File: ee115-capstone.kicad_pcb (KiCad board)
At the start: 4 copper layers, 191 parts, among them J1 2171790001, J2 9V_BATTERY, J3 Conn_01x04_Pin, J5 Conn_01x03_Pin, J6 Conn_02x02_Odd_Even, Q1 PMOS, Q2 NMOS, Q3 NPN, Q4 AO3400A, Q5 AO3400A, Q6 NMOS, Q7 PNP, Q8 NPN, SW1 SW_Push, SW2 SW_Push, SW3 SW_Push, U1 OPA2140AIDR, U10 SN74LVC1G02DCKR (NOR), U11 SN74LVC1G02DCKR (NOR), U12 ALD1107PBL, U13 LD39150DT33-R, U14 SL78L05, U15 300P14-U, U16 OPA705PA, U17 MIC4605-2YM-TR, U18 OPA705PA, U19 OPA705PA, U2 CD4052BPWR, U20 AD8038, U21 MCP6571T-E/OT, U3 LM393DR, U4 ADG601BRMZ-REEL7, U5 ESP32-C3-WROOM-02-N4, U6 AP2112K-3.3, U7 MCP601T-E_OT, U8 MCP6571T-E/OT, U9 MCP6571T-E/OT

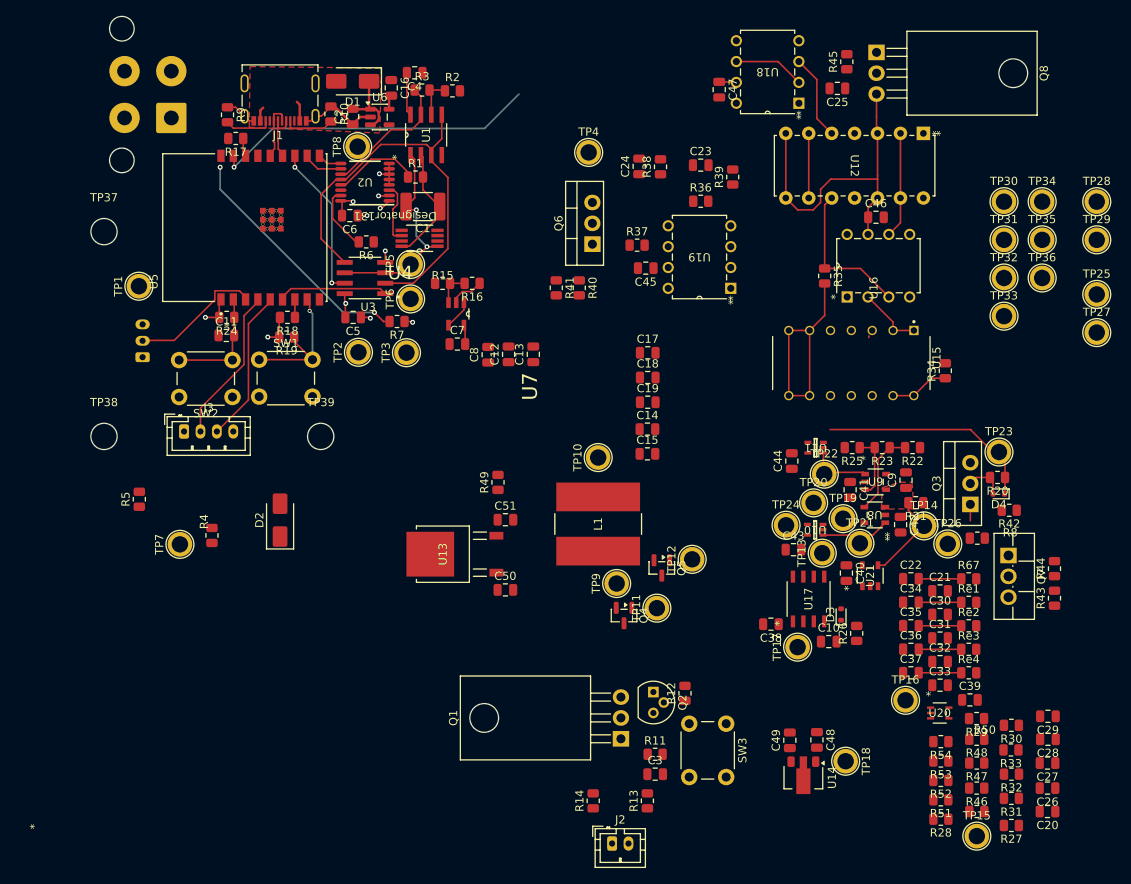
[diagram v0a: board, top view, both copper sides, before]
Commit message: pcb layout draft
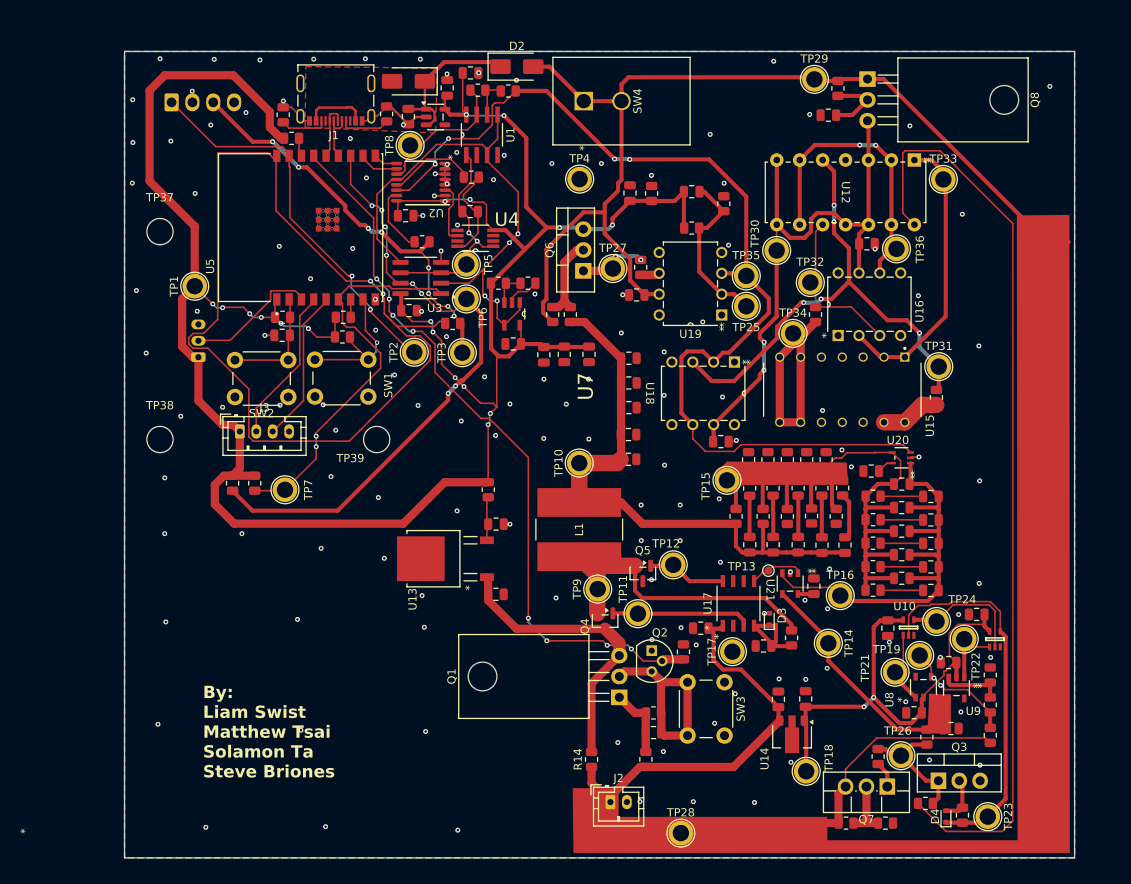
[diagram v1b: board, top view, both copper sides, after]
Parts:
- removed J6: Conn_02x02_Odd_Even, Connector_Molex:Molex_Mega-Fit_76829-0004_2x02_P5.70mm_Vertical
- removed TP20: TestPoint, TestPoint:TestPoint_Plated_Hole_D2.0mm
- added J4: Conn_01x04_Pin, Connector_Molex:Molex_KK-254_AE-6410-04A_1x04_P2.54mm_Vertical, B.Cu at (64.6, 100.4)
- added SW4: GF-123-0054, footprints_pretty:SW2_GF-123-0054_CWI, F.Cu at (114.8, 100.2)
- C1: footprint Capacitor_SMD:C_1812_4532Metric -> footprints_pretty:0805_cap_nosilk
- C10, C11, C12, C13, C14, C15, C16, C17, C18, C19, C2, C20, C21, C22, C23, C24, C25, C26, C27, C28, C29, C3, C30, C31, C32, C33, C34, C35, C36, C37, C38, C39, C4, C40, C41, C42, C43, C44, C45, C46, C47, C48, C49, C5, C50, C51, C6, C7, C8, C9: footprint Capacitor_SMD:C_0805_2012Metric -> footprints_pretty:0805_cap_nosilk
- R1, R10, R11, R12, R13, R15, R16, R17, R18, R19, R2, R20, R21, R22, R23, R24, R25, R26, R27, R28, R29, R3, R30, R31, R32, R33, R34, R35, R36, R37, R38, R39, R4, R40, R41, R42, R43, R44, R45, R46, R47, R48, R49, R5, R50, R51, R52, R53, R54, R6, R67, R7, R8, R9, Re1, Re2, Re3, Re4: footprint Resistor_SMD:R_0805_2012Metric -> footprints_pretty:res_0805_nosilk
- TP13: footprint TestPoint:TestPoint_Plated_Hole_D2.0mm -> TestPoint:TestPoint_Pad_D1.0mm
- moved TP28 92.1 mm to (126.7, 189.4)
- moved D2 62.3 mm to (106.7, 96.0), turned to 0 degrees
- moved TP27 59.5 mm to (118.4, 120.7)
- moved TP15 53.0 mm to (132.3, 146.5), turned to -90 degrees
- moved R27 50.4 mm to (133.4, 150.8), turned to 90 degrees
- moved R28 49.7 mm to (134.9, 143.9), turned to 90 degrees
- moved C20 48.7 mm to (135.1, 154.3), turned to 90 degrees
- moved R50 48.1 mm to (135.1, 147.4), turned to 90 degrees
- moved U18 47.4 mm to (125.6, 139.7), turned to -90 degrees
- moved R51 46.5 mm to (137.3, 143.9), turned to 90 degrees
- moved R31 45.8 mm to (136.7, 150.8), turned to 90 degrees
- moved C26 44.7 mm to (137.9, 154.3), turned to 90 degrees
- moved TP23 44.4 mm to (164.1, 187.4), turned to -90 degrees
- moved R46 44.2 mm to (137.9, 147.4), turned to 90 degrees
- moved R52 43.3 mm to (139.6, 143.9), turned to 90 degrees
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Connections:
- C12 pad 2: 3V3 -> +3V3
- C13 pad 2: 3V3 -> +3V3
- J3 pad 1: 3V3 -> +3V3
- R17 pad 2: 3V3 -> +3V3
- R18 pad 2: 3V3 -> +3V3
- R19 pad 2: 3V3 -> +3V3
- R24 pad 2: 3V3 -> +3V3
- TP35 pad 1: /Buck Converter/bg_volt -> /V_BG
- U18 pad 2: /Buck Converter/bg_volt -> /V_BG
- U18 pad 6: /Buck Converter/bg_volt -> /V_BG
- U19 pad 3: /Buck Converter/bg_volt -> /V_BG
- U20 pad 3: /Buck Converter/bg_volt -> /V_BG
- U5 pad 1: 3V3 -> +3V3
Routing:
- net +3V3: track 17.3 -> 289.7 mm, vias 3 -> 18
- net +9V: track 0.00 -> 255.7 mm
- net /V_BG: track 0.00 -> 126.0 mm, vias 0 -> 4
- net /Buck Converter/I_PTAT: track 0.00 -> 112.8 mm
- net /POWER_LATCH: track 0.00 -> 90.1 mm, vias 0 -> 8
- net /ADC-MCU/ESP_ADC_1: track 30.0 -> 117.6 mm
- net Net-(U20--): track 0.00 -> 74.5 mm
- net +3.5V: track 0.00 -> 70.7 mm
- net +5V: track 4.24 -> 67.6 mm, vias 0 -> 2
- net /ADC-MCU/COMP_OUT_BAR: track 18.9 -> 76.5 mm, vias 2 -> 8
- net /Buck Converter/error: track 0.00 -> 54.6 mm
- net /bandgap/vref: track 10.4 -> 61.2 mm, vias 0 -> 5
- net /Thermopile: track 1.03 -> 49.8 mm, vias 1 -> 8
- net /Buck Converter/switch_node: track 0.00 -> 39.7 mm
- net /ADC-MCU/COMP_OUT: track 13.5 -> 48.3 mm, vias 0 -> 2
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- added copper zone on B.Cu, net GND
- added copper zone on F.Cu, net GND
- removed copper zone on F.Cu, net /Buck Converter/Sawtooth Generator/saw
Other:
- board outline added: 115.8 x 98.2 mm
- board text added: "By: Liam Swist Matthew Tsai Solamon Ta Steve Briones"
